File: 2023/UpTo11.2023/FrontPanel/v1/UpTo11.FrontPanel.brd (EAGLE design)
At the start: 88 x 78 mm, 16 parts

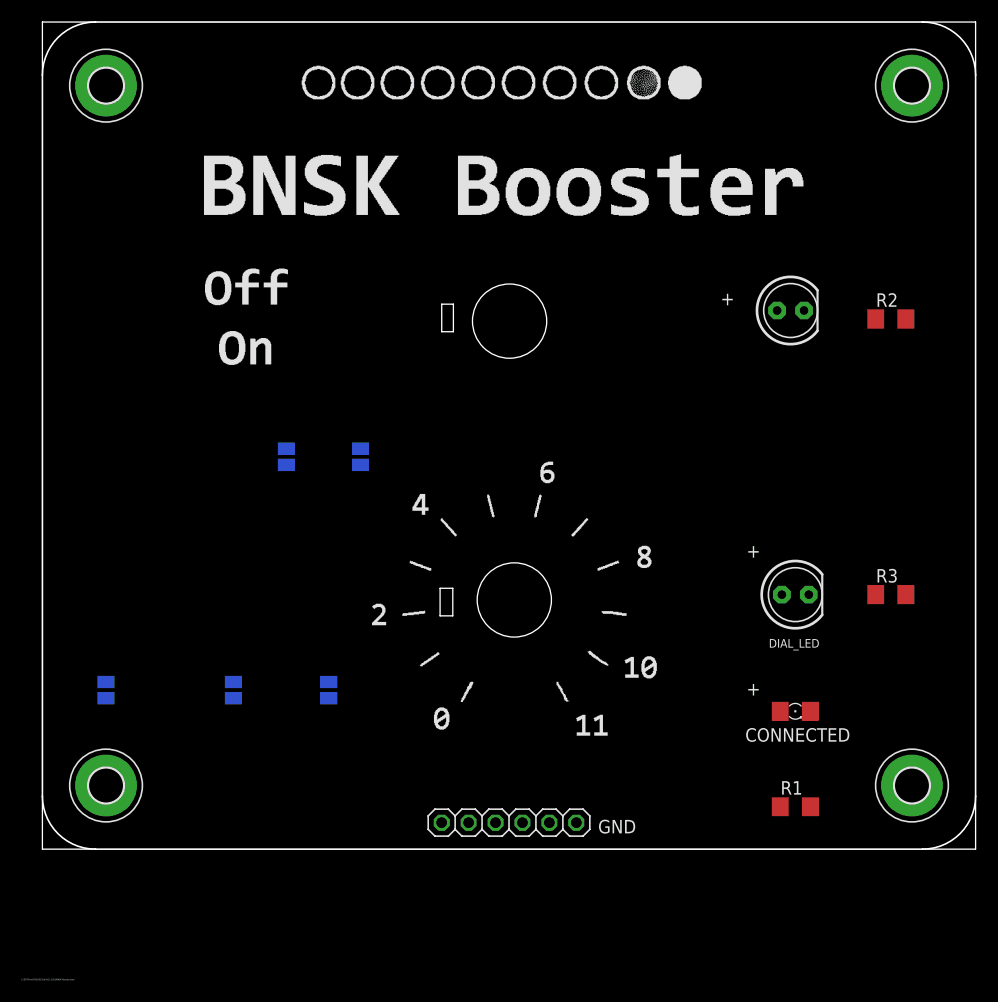
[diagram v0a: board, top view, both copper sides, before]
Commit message: BNSK Booster v 2
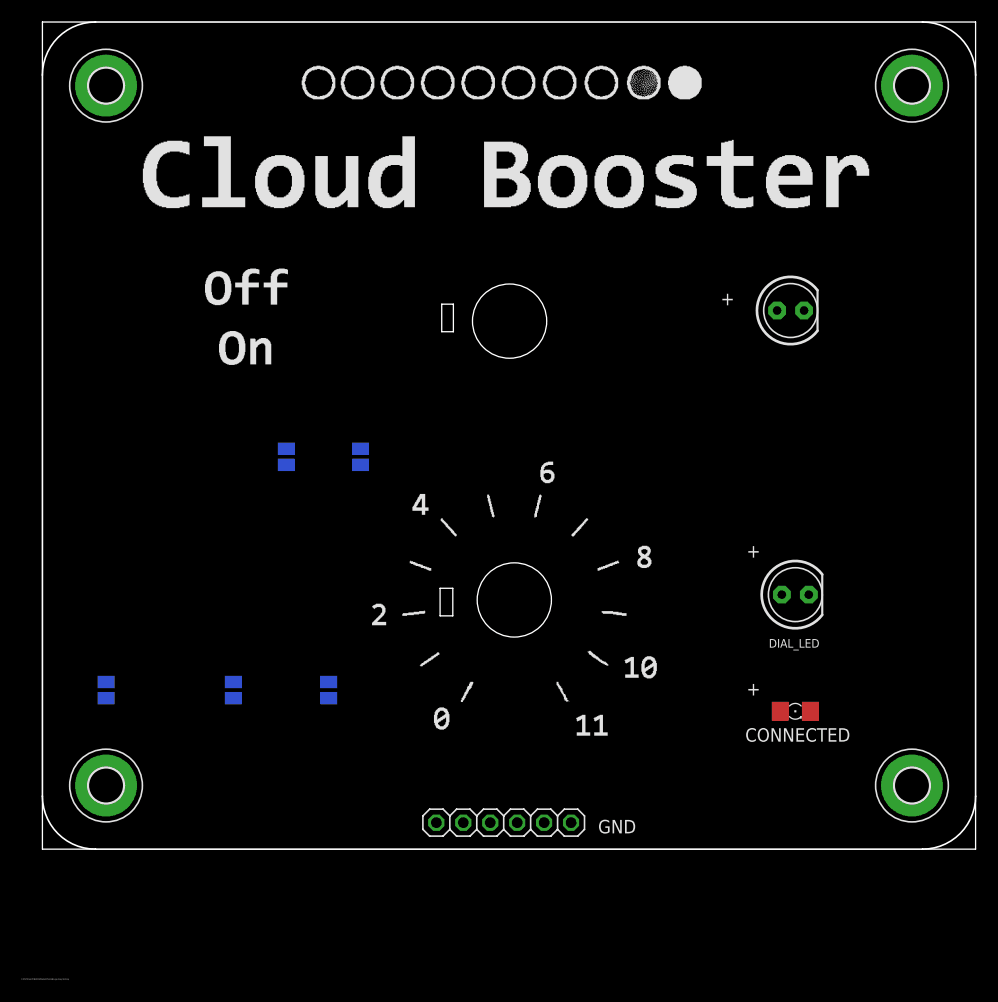
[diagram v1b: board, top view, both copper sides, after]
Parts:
- removed R1, R2, R3: (no value), adafruit:R1206
- moved FRONT_PANEL_INTERFACE 0.50 mm to (45.5, 14.5)
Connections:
- removed net N$1: CONNECTED.C, R1.2
- removed net N$2: BOOSTER_ON_LED.K, R2.2
- removed net N$3: DIAL_LED.K, R3.2
- new net VCC_1K: CONNECTED.A, FRONT_PANEL_INTERFACE.3, SWITCH_IN.2
- net GND_EX: now also BOOSTER_ON_LED.K, CONNECTED.C, DIAL_LED.K; no longer R1.1, R2.1, R3.1
- net VCC: now also FRONT_PANEL_INTERFACE.2; no longer CONNECTED.A, FRONT_PANEL_INTERFACE.6, SWITCH_IN.2
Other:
- board text added: "C:/DVT/Fred.PCB/2023/MadeInTheUSB.Logo.Gray.50.bmp"
- board text removed: "C:/DVT/Fred.PCB/2023/UpTo11.2023/BNSK Booster.bmp"
